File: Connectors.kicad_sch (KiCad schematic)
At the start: 12 parts, among them J4 Conn_02x03_Odd_Even, U12 TJA1051T/3

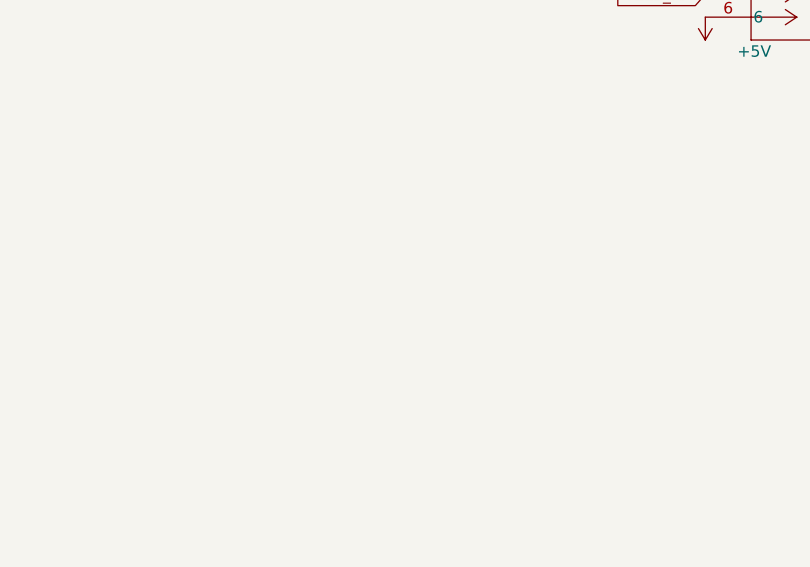
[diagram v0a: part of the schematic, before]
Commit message: update
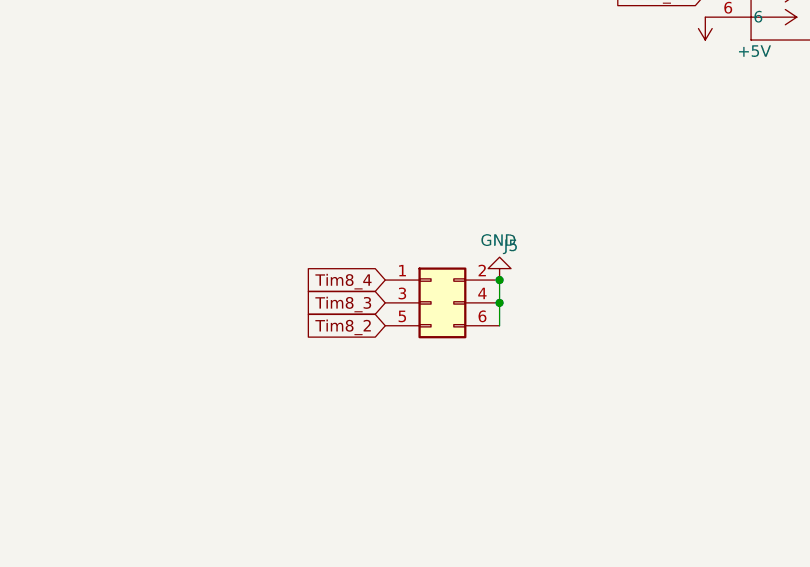
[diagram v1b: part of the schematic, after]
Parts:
- added J5: Conn_02x03_Odd_Even, Connector_PinSocket_2.00mm:PinSocket_2x03_P2.00mm_Vertical, symbol Connector_Generic:Conn_02x03_Odd_Even
- TELE1: footprint CONN_SM06B-GHS-TB_JST -> mylib:CONN_SM06B-GHS-TB_JST
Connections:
- net GND: now also J5.2 (Pin_2), J5.4 (Pin_4), J5.6 (Pin_6)
- new net Tim8_2: J5.5 (Pin_5)
- new net Tim8_3: J5.3 (Pin_3)
- new net Tim8_4: J5.1 (Pin_1)
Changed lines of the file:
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@@
+	)
+	(junction
+		(at 219.71 120.65)
+		(diameter 0)
+		(color 0 0 0 0)
 	)
 	(junction
@@
 		(color 0 0 0 0)
 	)
+	(junction
+		(at 219.71 123.19)
+		(diameter 0)
+		(color 0 0 0 0)
+	)
 	(polyline
 		(pts
@@
 	(wire
 		(pts
+			(xy 219.71 123.19) (xy 219.71 125.73)
+		)
+		(stroke
+			(width 0)
+			(type default)
+		)
+	)
+	(wire
+		(pts
 			(xy 80.01 40.64) (xy 80.01 41.91)
 		)
@@
 		(pts
 			(xy 77.47 40.64) (xy 62.23 40.64)
+		)
+		(stroke
+			(width 0)
+			(type default)
+		)
+	)
+	(wire
+		(pts
+			(xy 219.71 120.65) (xy 219.71 123.19)
 		)
 		(stroke
@@
 		)
 	)
+	(global_label "Tim8_4"
+		(shape input)
+		(at 207.01 120.65 180)
+		(effects
+			(font
+				(size 1.27 1.27)
+			)
+			(justify right)
+		)
+		(property "Intersheetrefs" "${INTERSHEET_REFS}"
+			(at 207.01 120.65 0)
+			(effects
+				(font
+					(size 1.27 1.27)
+				)
+				(hide yes)
+			)
+		)
+	)
 	(global_label "SWDIO"
 		(shape input)
@@
 		)
 	)
+	(global_label "Tim8_2"
+		(shape input)
+		(at 207.01 125.73 180)
+		(effects
+			(font
+				(size 1.27 1.27)
+			)
+			(justify right)
+		)
+		(property "Intersheetrefs" "${INTERSHEET_REFS}"
+			(at 207.01 125.73 0)
+			(effects
+				(font
+					(size 1.27 1.27)
+				)
+				(hide yes)
+			)
+		)
+	)
 	(global_label "GPS_RX"
 		(shape input)
@@
 		)
 	)
+	(global_label "Tim8_3"
+		(shape input)
+		(at 207.01 123.19 180)
+		(effects
+			(font
+				(size 1.27 1.27)
+			)
+			(justify right)
+		)
+		(property "Intersheetrefs" "${INTERSHEET_REFS}"
+			(at 207.01 123.19 0)
+			(effects
+				(font
+					(size 1.27 1.27)
+				)
+				(hide yes)
+			)
+		)
+	)
 	(symbol
 		(lib_id "power:GND")
@@
 			)
 		)
-		(property "Footprint" "CONN_SM06B-GHS-TB_JST"
+		(property "Footprint" "mylib:CONN_SM06B-GHS-TB_JST"
 			(at 242.57 78.74 0)
 			(effects
@@
 	)
 	(symbol
+		(lib_id "power:GND")
+		(at 219.71 120.65 180)
+		(unit 1)
+		(exclude_from_sim no)
+		(in_bom yes)
+		(on_board yes)
+		(dnp no)
+		(property "Reference" "#PWR015"
+			(at 219.71 114.3 0)
+			(effects
+				(font
+					(size 1.27 1.27)
+				)
+				(hide yes)
+			)
+		)
+		(property "Value" "GND"
+			(at 219.583 116.2558 0)
+			(effects
+				(font
+					(size 1.27 1.27)
+				)
+			)
+		)
+		(property "Footprint" ""
+			(at 219.71 120.65 0)
+			(effects
+				(font
+					(size 1.27 1.27)
+				)
+				(hide yes)
+			)
+		)
+		(property "Datasheet" ""
+			(at 219.71 120.65 0)
+			(effects
+				(font
+					(size 1.27 1.27)
+				)
+				(hide yes)
+			)
+		)
+		(property "Description" "Power symbol creates a global label with name \"GND\" , ground"
+			(at 219.71 120.65 0)
+			(effects
+				(font
+					(size 1.27 1.27)
+				)
+				(hide yes)
+			)
+		)
+		(pin "1"
+		)
+		(instances
+			(project "MX_IMU"
+				(path "/8ed38441-7d4e-4e89-870f-07e11c6dce38/3e6b1080-2480-49a7-8bae-2dbfae5f98f5"
+					(reference "#PWR015")
+					(unit 1)
+				)
+			)
+		)
+	)
+	(symbol
 		(lib_id "power:+5V")
 		(at 201.93 58.42 0)
@@
 					(unit 1)
 				)
+			)
+		)
+	)
+	(symbol
+		(lib_id "Connector_Generic:Conn_02x03_Odd_Even")
+		(at 212.09 123.19 0)
+		(unit 1)
+		(exclude_from_sim no)
+		(in_bom yes)
+		(on_board yes)
+		(dnp no)
+		(property "Reference" "J5"
+			(at 220.98 116.84 0)
+			(effects
+				(font
+					(size 1.27 1.27)
+				)
+			)
+		)
+		(property "Value" "Conn_02x03_Odd_Even"
+			(at 213.36 116.84 0)
+			(effects
+				(font
+					(size 1.27 1.27)
+				)
+				(hide yes)
+			)
+		)
+		(property "Footprint" "Connector_PinSocket_2.00mm:PinSocket_2x03_P2.00mm_Vertical"
+			(at 212.09 123.19 0)
+			(effects
+				(font
+					(size 1.27 1.27)
+				)
+				(hide yes)
+			)
+		)
+		(property "Datasheet" "~"
+			(at 212.09 123.19 0)
+			(effects
+				(font
+					(size 1.27 1.27)
+				)
+				(hide yes)
+			)
+		)
+		(property "Description" "Generic connector, double row, 02x03, odd/even pin numbering scheme (row 1 odd numbers, row 2 even numbers), script generated (kicad-library-utils/schlib/autogen/connector/)"
+			(at 212.09 123.19 0)
+			(effects
+				(font
+					(size 1.27 1.27)
+				)
+				(hide yes)
+			)
+		)
+		(pin "6"
+		)
+		(pin "1"
+		)
+		(pin "4"
+		)
+		(pin "3"
+		)
+		(pin "2"
+		)
+		(pin "5"
+		)
+		(instances
+			(project "MX_IMU"
+				(path "/8ed38441-7d4e-4e89-870f-07e11c6dce38/3e6b1080-2480-49a7-8bae-2dbfae5f98f5"
+					(reference "J5")
+					(unit 1)
+				)
